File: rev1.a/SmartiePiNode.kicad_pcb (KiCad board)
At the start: 2 copper layers, 71.7 x 55 mm, 52 parts, among them CN1 USBMICROb, CN2 ST-LINK, CN3 SX1238_TRX_HEADER, SW1 SW_PUSH, U1 ISL91127IR, U2 STM32L052_LQFP48, X1 abm10, X2 ABS25-32.768KHZ-6-T

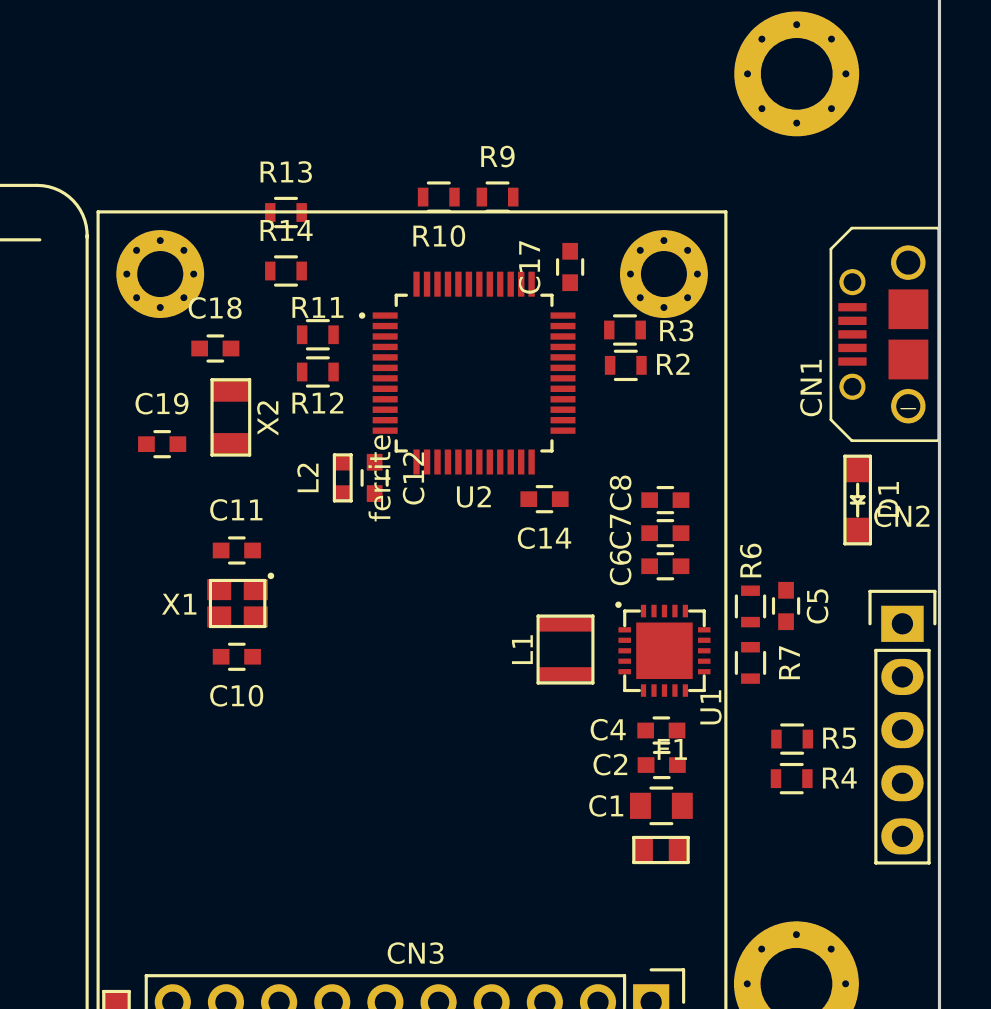
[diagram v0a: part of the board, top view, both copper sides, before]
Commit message: more placement and layout.
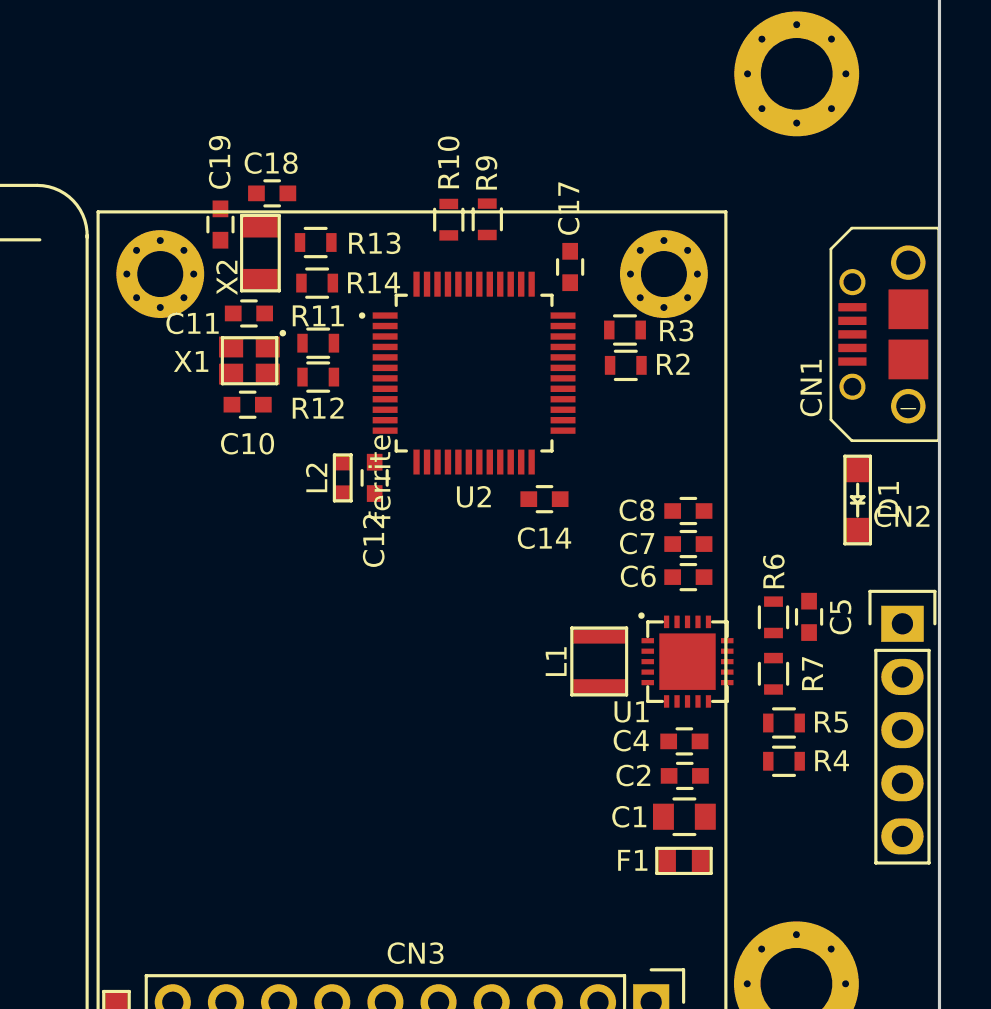
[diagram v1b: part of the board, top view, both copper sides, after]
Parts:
- moved C10 12.1 mm to (137.7, 117.2)
- moved X1 11.6 mm to (137.8, 115.1)
- moved C11 11.3 mm to (137.8, 112.9)
- moved C19 10.9 mm to (136.4, 108.6), turned to 270 degrees
- moved X2 7.97 mm to (138.3, 110.0)
- moved C18 7.90 mm to (138.9, 107.1), turned to 180 degrees
- moved R13 2.02 mm to (140.9, 109.5)
- moved L1 1.71 mm to (154.5, 129.5)
- moved R14 1.60 mm to (141.0, 111.4)
- moved U1 1.22 mm to (158.7, 129.5)
- moved C1 1.22 mm to (158.6, 136.9)
- moved C4 1.22 mm to (158.6, 133.3)
- moved C7 1.22 mm to (158.7, 123.9)
- moved C8 1.22 mm to (158.7, 122.3)
- moved R6 1.22 mm to (162.8, 127.4)
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
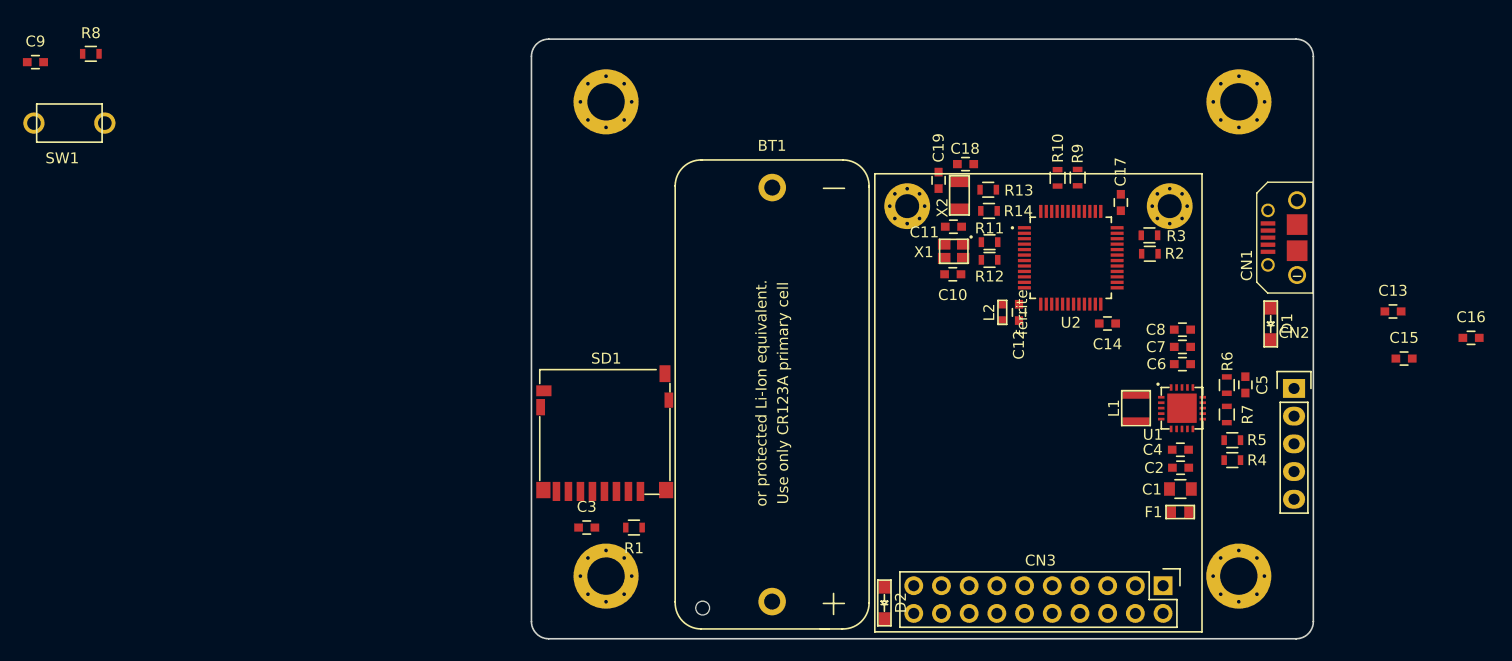
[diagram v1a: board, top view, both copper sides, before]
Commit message: more layout
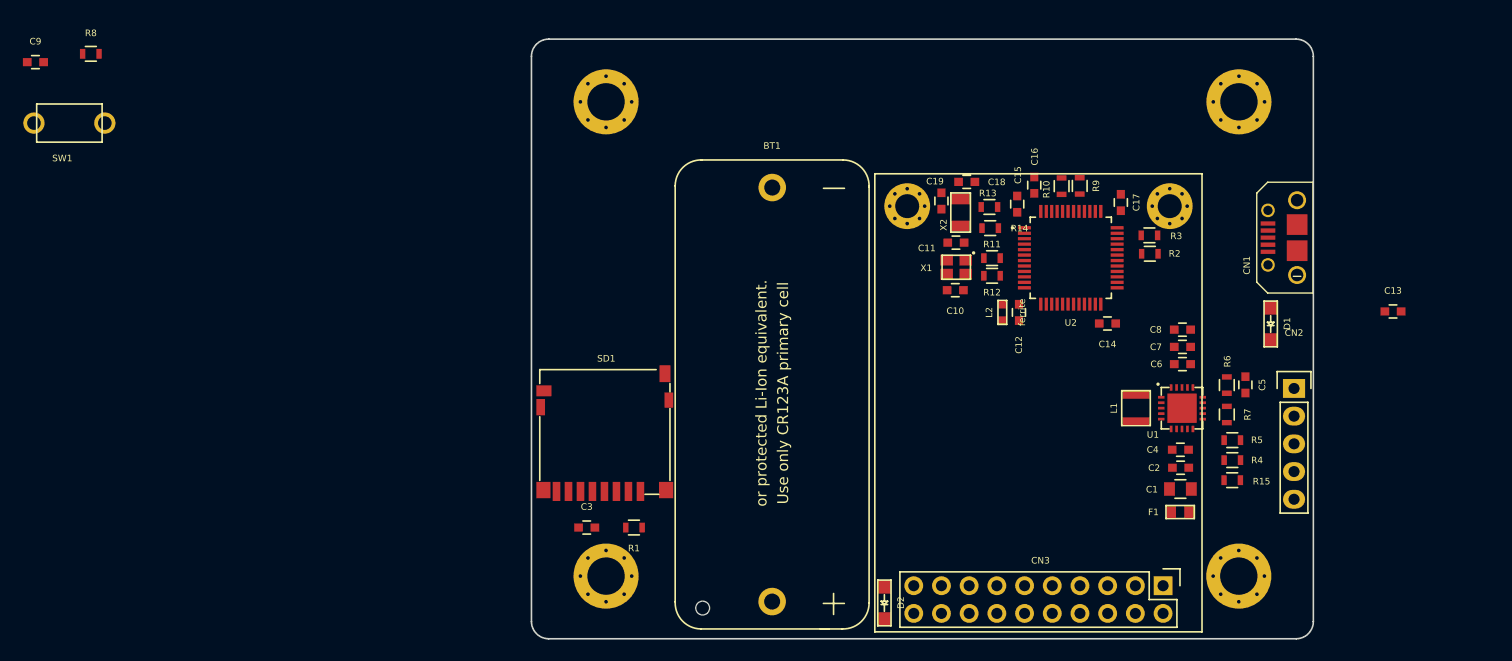
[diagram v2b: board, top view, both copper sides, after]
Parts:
- added R15: 10K, Resistors_SMD:R_0603, F.Cu at (163.3, 136.1)
- R4: value 0 -> 10K
- moved C16 42.4 mm to (145.2, 109.1), turned to 90 degrees
- moved C15 38.2 mm to (143.6, 110.8), turned to 90 degrees
- moved C19 1.91 mm to (136.7, 110.5)
- moved C18 1.63 mm to (139.0, 108.8)
- moved R13 1.58 mm to (141.1, 111.1)
- moved R14 1.58 mm to (141.1, 113.0)
- moved X2 1.58 mm to (138.4, 111.6)
- moved C10 1.48 mm to (137.9, 118.7)
- moved C11 1.48 mm to (138.0, 114.3)
- moved R11 1.48 mm to (141.3, 115.8)
- moved X1 1.48 mm to (138.0, 116.6)
- moved R12 1.48 mm to (141.3, 117.4)
- moved R10 0.85 mm to (147.7, 109.2)
- moved R9 0.78 mm to (149.3, 109.1)
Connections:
- U1 pad 11: /+VIN -> Net-(R15-Pad1)
